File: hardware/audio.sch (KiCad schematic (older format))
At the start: 24 parts, among them U4 FM8002A, U5 TM8211, U6 FM8002A

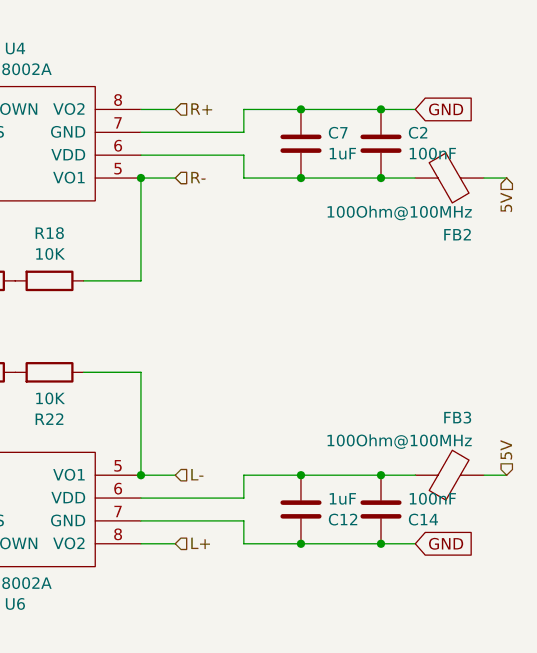
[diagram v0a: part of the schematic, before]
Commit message: Dumb leds and stm32 magic
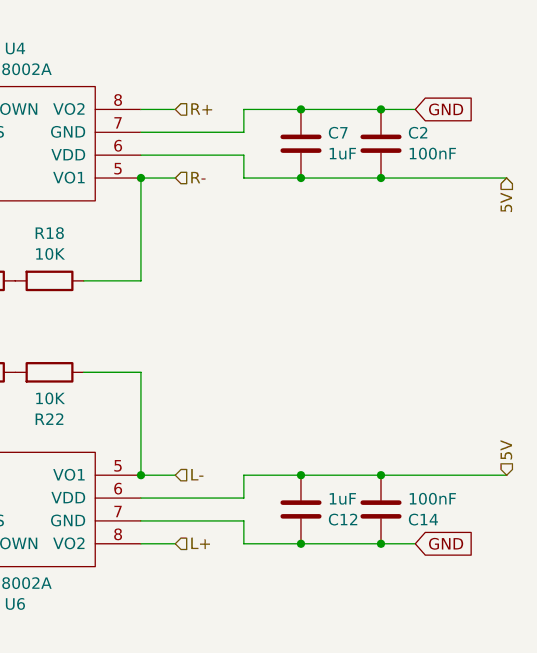
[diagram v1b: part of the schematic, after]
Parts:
- removed FB2, FB3: 100Ohm@100MHz, Inductor_SMD:L_0603_1608Metric, symbol Device:Ferrite_Bead
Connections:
- net 5V: now also C12.1, C14.1, C2.1, C7.1, U4.6 (VDD), U6.6 (VDD)
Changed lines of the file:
@@
 EESchema Schematic File Version 4
-LIBS:cz-badge-hardware-cache
 EELAYER 30 0
 EELAYER END
 $Descr A4 11693 8268
 encoding utf-8
-Sheet 3 3
+Sheet 3 5
 Title ""
 Date ""
@@
 $EndComp
 Connection ~ 6500 2600
-Wire Wire Line
-	6500 2600 6650 2600
 Connection ~ 6500 2300
 Wire Wire Line
@@
 $EndComp
 Connection ~ 6500 3900
-Wire Wire Line
-	6500 3900 6650 3900
 Connection ~ 6500 4200
 Wire Wire Line
@@
 	2400 3550 2200 3550
 Connection ~ 2400 3550
-Wire Wire Line
-	7050 3900 6950 3900
 Text HLabel 7050 3900 1    50   Input ~ 0
 5V
-$Comp
-L Device:Ferrite_Bead FB3
-U 1 1 5DFCD30D
-P 6800 3900
-F 0 "FB3" V 7050 3800 50  0000 L CNN
-F 1 "100Ohm@100MHz" V 6950 3800 50  0000 L CNN
-F 2 "Inductor_SMD:L_0603_1608Metric" V 6730 3900 50  0001 C CNN
-F 3 "~" H 6800 3900 50  0001 C CNN
-	1    6800 3900
-	0    -1   -1   0
-$EndComp
 Text HLabel 7050 2600 3    50   Input ~ 0
 5V
-$Comp
-L Device:Ferrite_Bead FB2
-U 1 1 5DFD1FD3
-P 6800 2600
-F 0 "FB2" V 7050 2500 50  0000 L CNN
-F 1 "100Ohm@100MHz" V 6950 2500 50  0000 L CNN
-F 2 "Inductor_SMD:L_0603_1608Metric" V 6730 2600 50  0001 C CNN
-F 3 "~" H 6800 2600 50  0001 C CNN
-	1    6800 2600
-	0    -1   1    0
-$EndComp
-Wire Wire Line
-	6950 2600 7050 2600
+Wire Wire Line
+	6500 3900 7050 3900
+Wire Wire Line
+	6500 2600 7050 2600
 $EndSCHEMATC

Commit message: Added lcsc partnumbers
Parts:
- C10: LCSC (none) -> C16780
- C11, C14, C2: LCSC (none) -> C14663
- C12, C13, C5, C7: LCSC (none) -> C15849
- R13, R15, R19, R20: LCSC (none) -> C23186
- R16, R18, R21, R22: LCSC (none) -> C25804
- U4, U6: LCSC (none) -> C94625
- U5: LCSC (none) -> C92003
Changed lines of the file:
@@
 F 2 "Package_SO:SSOP-8_3.9x5.05mm_P1.27mm" H 1900 3500 50  0001 C CNN
 F 3 "" H 1900 3500 50  0001 C CNN
+F 4 "C92003" H 1900 3250 50  0001 C CNN "LCSC"
 	1    1900 3250
 	1    0    0    -1
@@
 F 2 "Package_SO:SSOP-8_3.9x5.05mm_P1.27mm" H 4850 2650 50  0001 C CNN
 F 3 "" H 4850 2650 50  0001 C CNN
+F 4 "C94625" H 4850 2400 50  0001 C CNN "LCSC"
 	1    4850 2400
 	1    0    0    -1
@@
 F 2 "Resistor_SMD:R_0603_1608Metric" V 4980 3050 50  0001 C CNN
 F 3 "~" H 5050 3050 50  0001 C CNN
+F 4 "C25804" H 5050 3050 50  0001 C CNN "LCSC"
 	1    5050 3050
 	0    1    1    0
@@
 F 2 "Resistor_SMD:R_0603_1608Metric" V 4680 3050 50  0001 C CNN
 F 3 "~" H 4750 3050 50  0001 C CNN
+F 4 "C25804" H 4750 3050 50  0001 C CNN "LCSC"
 	1    4750 3050
 	0    1    1    0
@@
 F 2 "Capacitor_SMD:C_0603_1608Metric" H 6188 2300 50  0001 C CNN
 F 3 "~" H 6150 2450 50  0001 C CNN
+F 4 "C15849" H 6150 2450 50  0001 C CNN "LCSC"
 	1    6150 2450
 	-1   0    0    1
@@
 F 2 "Capacitor_SMD:C_0603_1608Metric" H 4138 2250 50  0001 C CNN
 F 3 "~" H 4100 2400 50  0001 C CNN
+F 4 "C15849" H 4100 2400 50  0001 C CNN "LCSC"
 	1    4100 2400
 	0    -1   -1   0
@@
 F 2 "Resistor_SMD:R_0603_1608Metric" V 3930 3050 50  0001 C CNN
 F 3 "~" H 4000 3050 50  0001 C CNN
+F 4 "C23186" H 4000 3050 50  0001 C CNN "LCSC"
 	1    4000 3050
 	0    1    1    0
@@
 F 2 "Resistor_SMD:R_0603_1608Metric" V 3630 3050 50  0001 C CNN
 F 3 "~" H 3700 3050 50  0001 C CNN
+F 4 "C23186" H 3700 3050 50  0001 C CNN "LCSC"
 	1    3700 3050
 	0    1    1    0
@@
 F 2 "Package_SO:SSOP-8_3.9x5.05mm_P1.27mm" H 4850 4350 50  0001 C CNN
 F 3 "" H 4850 4350 50  0001 C CNN
+F 4 "C94625" H 4850 4100 50  0001 C CNN "LCSC"
 	1    4850 4100
 	1    0    0    1
@@
 F 2 "Resistor_SMD:R_0603_1608Metric" V 4980 3450 50  0001 C CNN
 F 3 "~" H 5050 3450 50  0001 C CNN
+F 4 "C25804" H 5050 3450 50  0001 C CNN "LCSC"
 	1    5050 3450
 	0    1    -1   0
@@
 F 2 "Resistor_SMD:R_0603_1608Metric" V 4680 3450 50  0001 C CNN
 F 3 "~" H 4750 3450 50  0001 C CNN
+F 4 "C25804" H 4750 3450 50  0001 C CNN "LCSC"
 	1    4750 3450
 	0    1    -1   0
@@
 F 2 "Capacitor_SMD:C_0603_1608Metric" H 6188 3900 50  0001 C CNN
 F 3 "~" H 6150 4050 50  0001 C CNN
+F 4 "C15849" H 6150 4050 50  0001 C CNN "LCSC"
 	1    6150 4050
 	-1   0    0    -1
@@
 F 2 "Capacitor_SMD:C_0603_1608Metric" H 4138 3950 50  0001 C CNN
 F 3 "~" H 4100 4100 50  0001 C CNN
+F 4 "C15849" H 4100 4100 50  0001 C CNN "LCSC"
 	1    4100 4100
 	0    -1   1    0
@@
 F 2 "Resistor_SMD:R_0603_1608Metric" V 3930 3450 50  0001 C CNN
 F 3 "~" H 4000 3450 50  0001 C CNN
+F 4 "C23186" H 4000 3450 50  0001 C CNN "LCSC"
 	1    4000 3450
 	0    1    -1   0
@@
 F 2 "Resistor_SMD:R_0603_1608Metric" V 3630 3450 50  0001 C CNN
 F 3 "~" H 3700 3450 50  0001 C CNN
+F 4 "C23186" H 3700 3450 50  0001 C CNN "LCSC"
 	1    3700 3450
 	0    1    -1   0
@@
 F 2 "Capacitor_SMD:C_0603_1608Metric" H 2038 3700 50  0001 C CNN
 F 3 "~" H 2000 3850 50  0001 C CNN
+F 4 "C14663" H 2000 3850 50  0001 C CNN "LCSC"
 	1    2000 3850
 	1    0    0    -1
@@
 F 2 "Capacitor_SMD:C_0805_2012Metric" H 1838 3700 50  0001 C CNN
 F 3 "~" H 1800 3850 50  0001 C CNN
+F 4 "C16780" H 1800 3850 50  0001 C CNN "LCSC"
 	1    1800 3850
 	1    0    0    -1
@@
 F 2 "Capacitor_SMD:C_0603_1608Metric" H 6538 2300 50  0001 C CNN
 F 3 "~" H 6500 2450 50  0001 C CNN
+F 4 "C14663" H 6500 2450 50  0001 C CNN "LCSC"
 	1    6500 2450
 	-1   0    0    1
@@
 F 2 "Capacitor_SMD:C_0603_1608Metric" H 6538 3900 50  0001 C CNN
 F 3 "~" H 6500 4050 50  0001 C CNN
+F 4 "C14663" H 6500 4050 50  0001 C CNN "LCSC"
 	1    6500 4050
 	-1   0    0    -1
